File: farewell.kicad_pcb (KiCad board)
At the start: 2 copper layers, 211 x 72 mm, 43 parts, among them U1 0

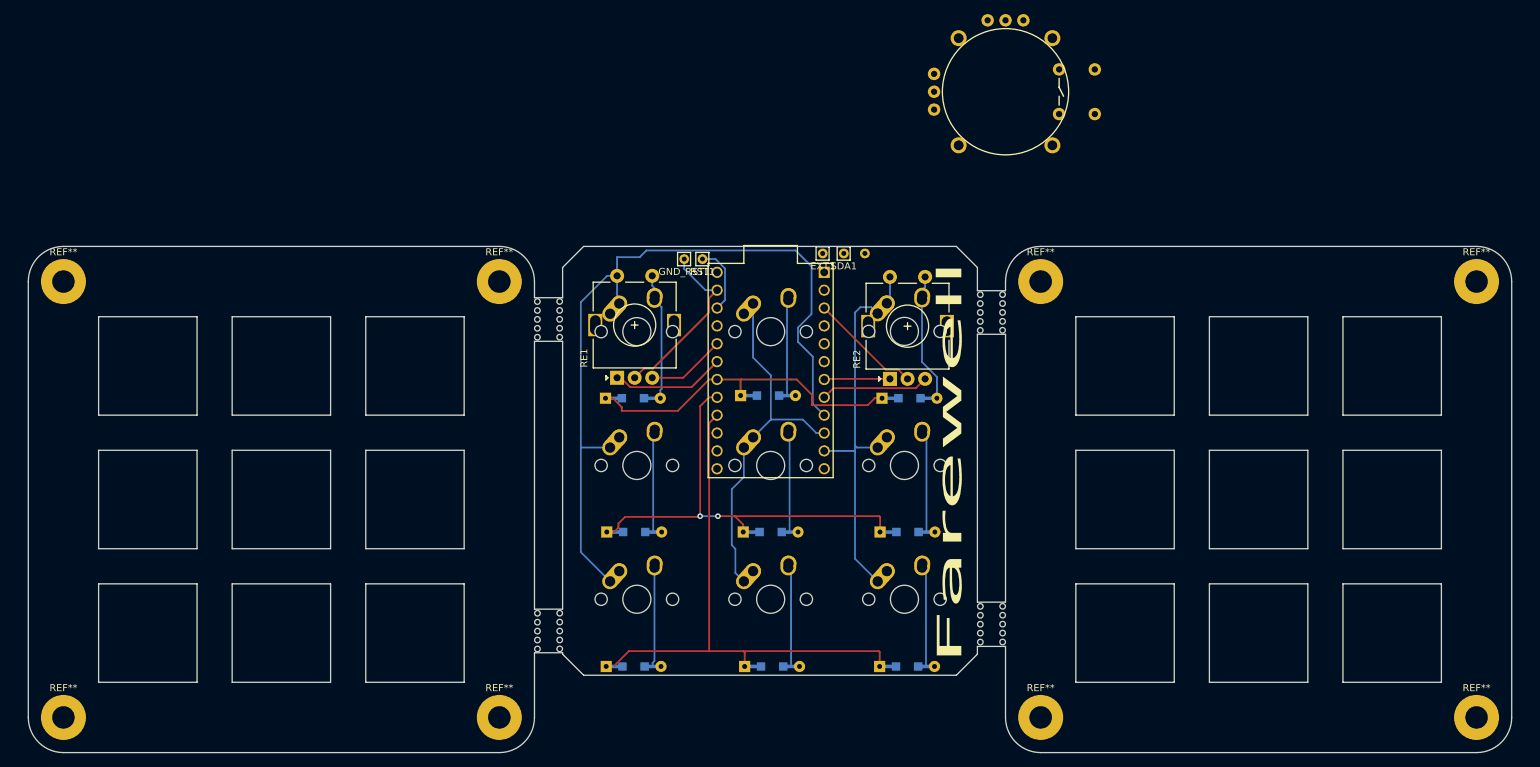
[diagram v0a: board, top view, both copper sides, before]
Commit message: farewell v1 pcb
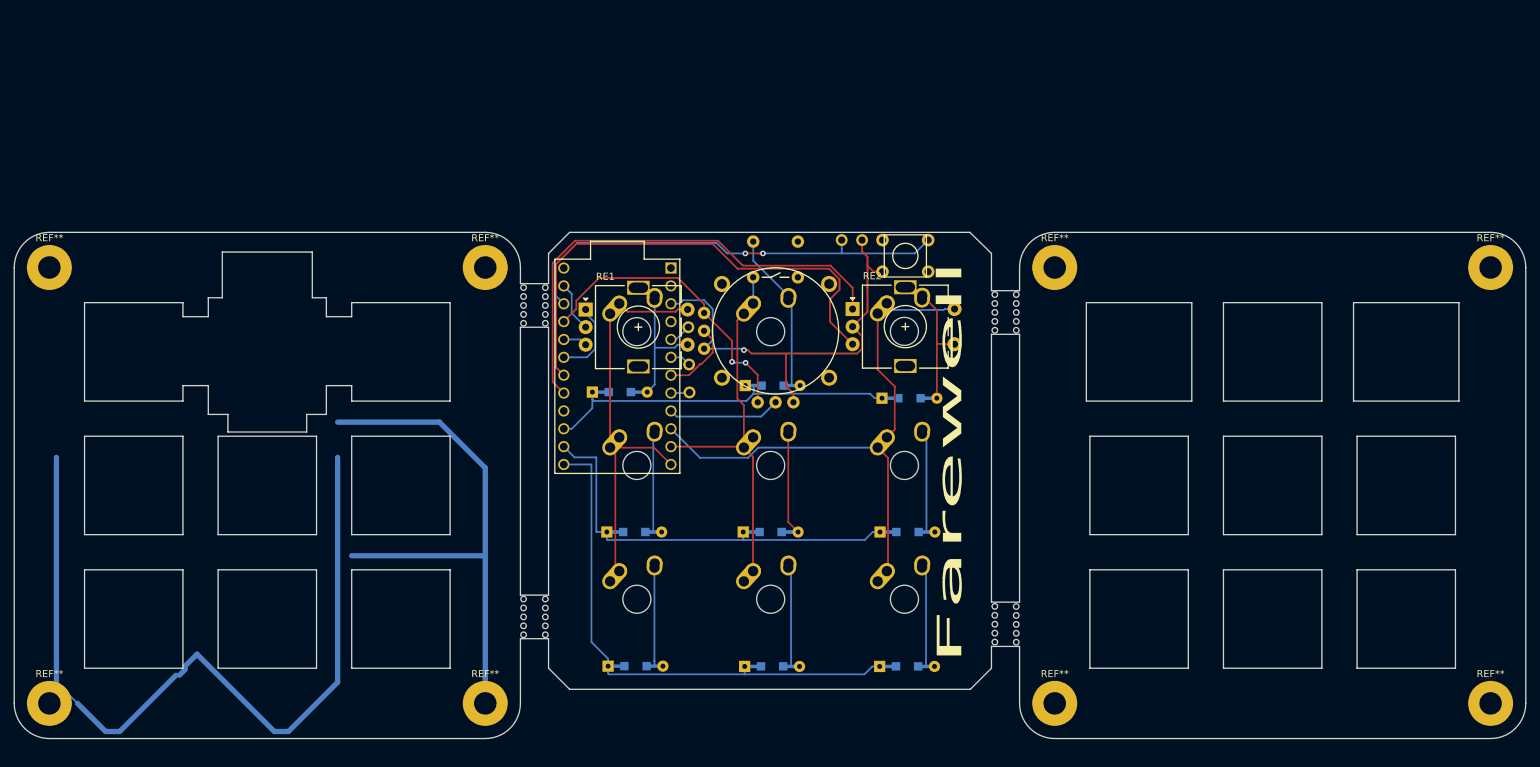
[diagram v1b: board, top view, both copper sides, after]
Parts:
- removed the REF** at (149.2, 50.4)
- removed the REF** at (152.3, 50.4)
- removed the REF** at (149.2, 94.7)
- removed the REF** at (152.3, 94.7)
- removed the REF** at (86.2, 51.4)
- removed the REF** at (89.3, 51.4)
- removed the REF** at (86.2, 95.7)
- removed the REF** at (89.3, 95.7)
- removed RST1: Conn_01x01, pin:Pin_D0.7mm_L6.5mm_W1.8mm_FlatFork
- added P?: CONN_1, keyboard_parts:PIN_1, F.Cu at (129.7, 40.1)
- added REF**: breakaway-mousebites, random-kb-part:breakaway-mousebites, F.Cu at (87.8, 93.7)
- added REF**: breakaway-mousebites, random-kb-part:breakaway-mousebites, F.Cu at (84.7, 93.7)
- added REF**: breakaway-mousebites, random-kb-part:breakaway-mousebites, F.Cu at (84.7, 49.4)
- added REF**: breakaway-mousebites, random-kb-part:breakaway-mousebites, F.Cu at (87.8, 49.4)
- added REF**: breakaway-mousebites, random-kb-part:breakaway-mousebites, F.Cu at (151.7, 50.4)
- added REF**: breakaway-mousebites, random-kb-part:breakaway-mousebites, F.Cu at (154.8, 50.4)
- added REF**: breakaway-mousebites, random-kb-part:breakaway-mousebites, F.Cu at (151.7, 94.7)
- added REF**: breakaway-mousebites, random-kb-part:breakaway-mousebites, F.Cu at (154.8, 94.8)
- added SW1: SW_Push, random-kb-part:PushButton_6x6mm_TH_Pretty, F.Cu at (138.8, 42.4)
- EXT1, GND_RST1, SCL1, SDA1: footprint pin:Pin_D0.7mm_L6.5mm_W1.8mm_FlatFork -> keyboard_parts:PIN_1
- MX1, MX2, MX3, MX4, MX5, MX6, MX7, MX8, MX9: footprint MX_Alps_Hybrid:MX-1U-NoLED -> farewell:MX-1U-NoLED-NoPCBMount
- moved JOY1 47.2 mm to (120.3, 53.0), turned to 0 degrees
- moved SCL1 29.6 mm to (108.0, 57.8)
- moved EXT1 27.4 mm to (108.0, 61.8)
- moved GND_RST1 25.4 mm to (132.6, 40.1)
- moved SDA1 24.5 mm to (107.9, 52.5)
- moved U1 21.8 mm to (97.8, 58.0)
- moved RE2 11.3 mm to (131.2, 49.9), turned to 0 degrees
- moved RE1 10.7 mm to (93.3, 50.0), turned to 0 degrees
- moved REF** 2.83 mm to (17.0, 106.0)
- moved REF** 2.83 mm to (17.0, 44.0)
- moved REF** 2.83 mm to (79.0, 44.0)
- moved REF** 2.83 mm to (160.0, 106.0)
- moved REF** 2.83 mm to (222.0, 106.0)
- moved REF** 2.83 mm to (222.0, 44.0)
- moved REF** 2.83 mm to (160.0, 44.0)
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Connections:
- GND_RST1 pad 1: E_G1 -> E_G2
- JOY1 pad H3: E_G1 -> E_G2
- JOY1 pad V3: E_G1 -> E_G2
- U1 pad 10: COL1 -> COL2
- U1 pad 11: COL2 -> COL1
- U1 pad 12: Net-(EXT1-Pad1) -> COL0
- U1 pad 17: ADC2 -> E2A
- U1 pad 18: ADC1 -> E2B
- U1 pad 7: E2A -> ADC1
- U1 pad 8: E2B -> Net-(EXT1-Pad1)
- U1 pad 9: COL0 -> ADC2
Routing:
- net (no net): track 0.00 -> 195.4 mm
- net E2A: track 9.38 -> 68.9 mm
- net E2B: track 15.4 -> 71.0 mm
- net Net-(SW1-Pad1): track 9.84 -> 63.6 mm, vias 0 -> 2
- net COL0: track 113.3 -> 60.7 mm
- net E_G2: track 16.0 -> 63.2 mm, vias 0 -> 1
- net VCC: track 0.00 -> 42.9 mm, vias 0 -> 2
- net COL2: track 55.2 -> 82.2 mm
- net E_G1: track 25.4 -> 7.15 mm
- net ADC2: track 0.00 -> 16.1 mm
- net ADC1: track 0.00 -> 10.9 mm
- net JOY_SW_1: track 13.7 -> 22.7 mm
- net E1B: track 11.2 -> 3.42 mm
- net E1A: track 16.3 -> 11.1 mm
- net ROW1: track 63.7 -> 58.9 mm, vias 2 -> 0
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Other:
- board size 211 x 72 mm -> 215 x 72 mm
- board text added: "GND"
- board text added: "PWM"
- board text added: "RST"
- board text added: "SCL"
- board text added: "SDA"
